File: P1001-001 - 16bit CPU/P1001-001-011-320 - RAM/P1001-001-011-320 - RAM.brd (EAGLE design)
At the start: 200 x 100 mm, 46 parts, among them IC1 74ALS21D, IC10 74ALS08D, IC2 74283D, IC27 MEGA8535-A, IC3 74ALS04D, IC4 74ALS02D, IC5 74LS32D, IC6 74283D, IC7 74283D, IC8 74283D, IC9 74LS32D

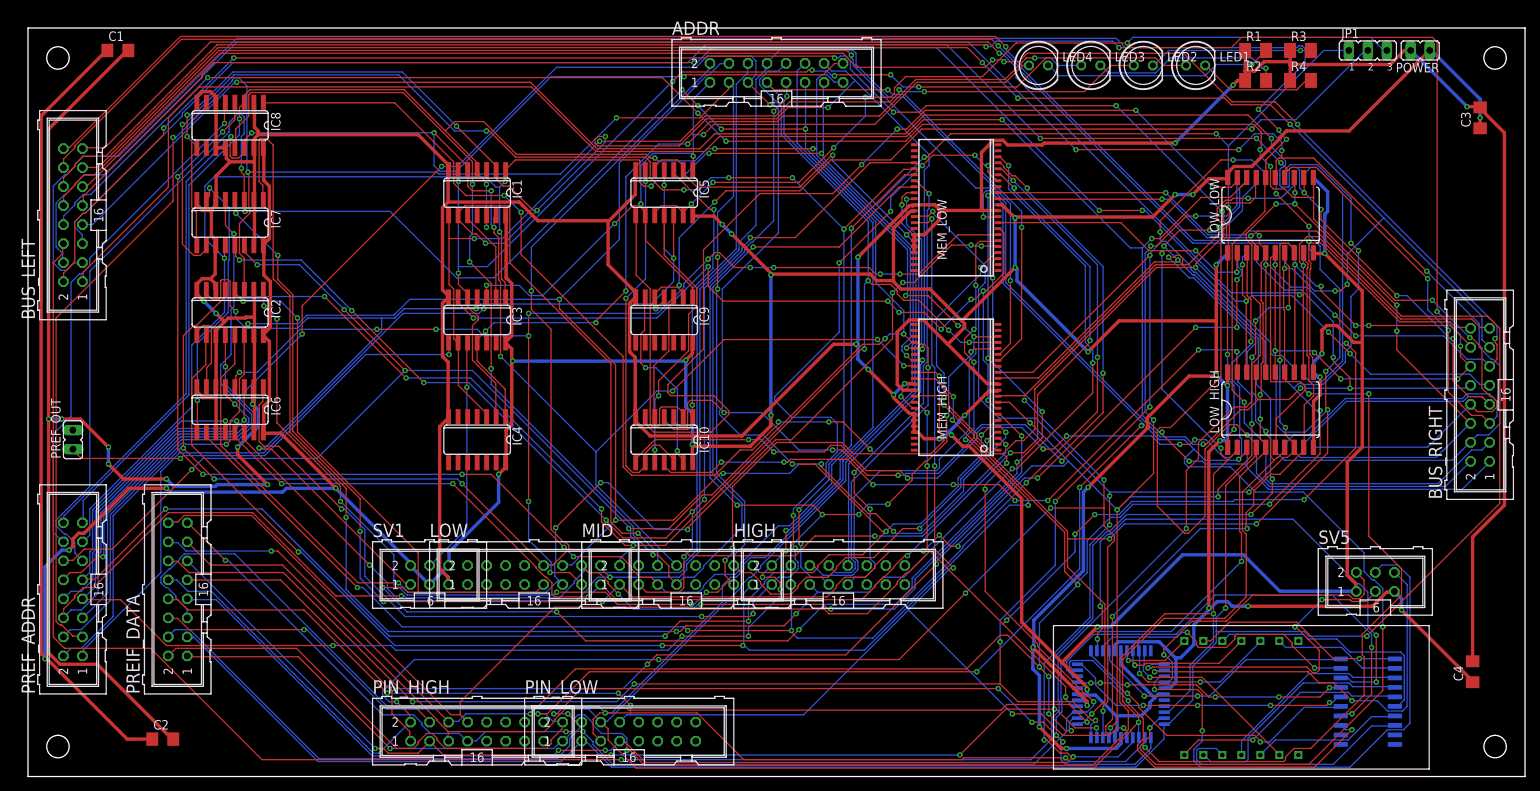
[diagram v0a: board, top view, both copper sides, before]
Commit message: Add the prototype stuff
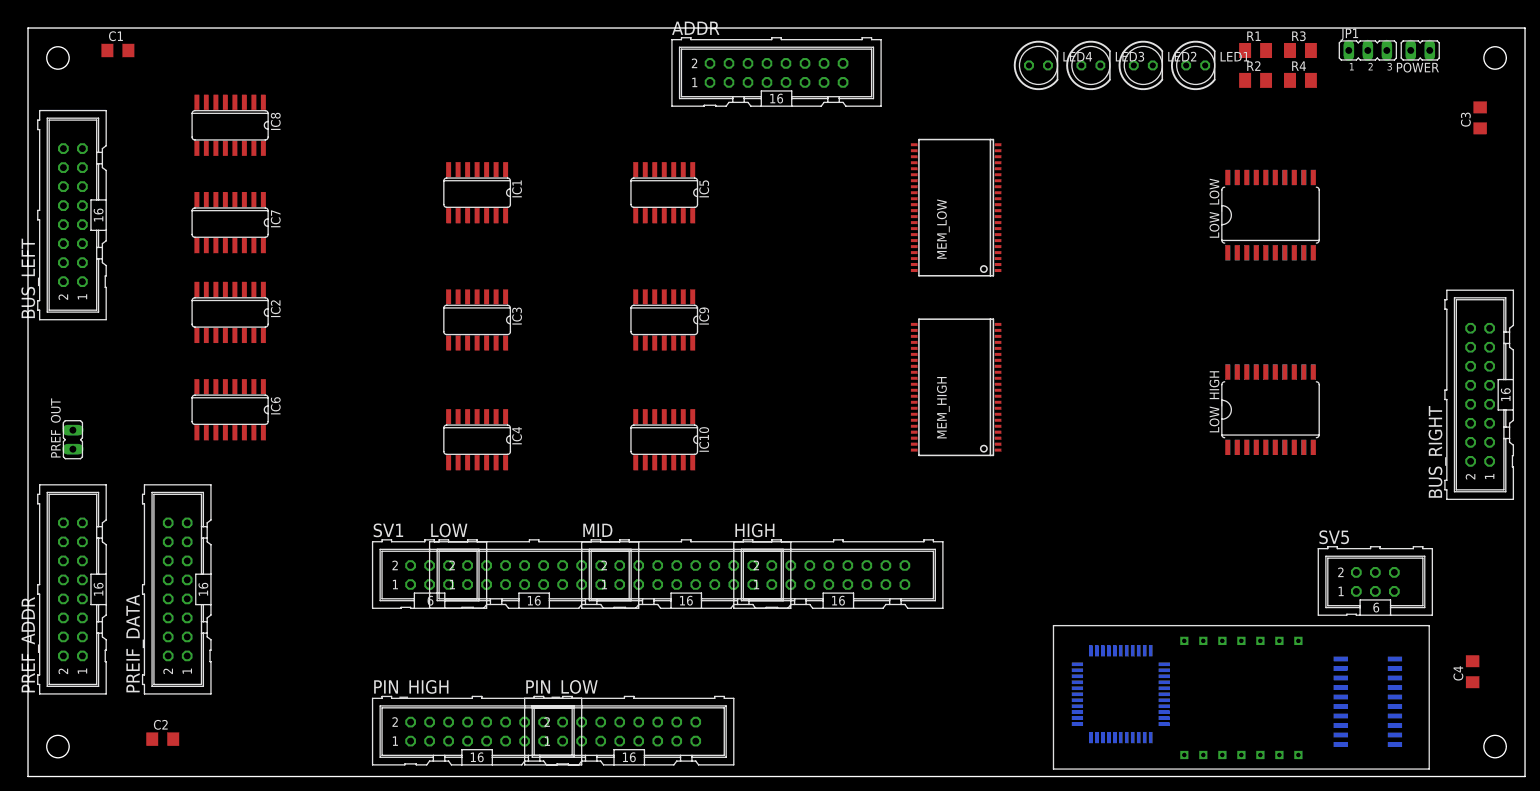
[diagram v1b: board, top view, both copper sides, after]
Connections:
- removed net LOWADDR1: IC2.4, LOW.9, MEM_LOW.3
- removed net LOWADDR10: HIGH.5, IC7.1, MEM_LOW.20
- removed net LOWADDR11: IC7.13, MEM_LOW.26, MID.3
- removed net LOWADDR12: HIGH.7, IC7.10, MEM_LOW.27
- removed net LOWADDR13: IC8.4, MEM_LOW.28, MID.5
- removed net LOWADDR14: HIGH.9, IC8.1, MEM_LOW.29
- removed net LOWADDR15: IC8.13, MEM_LOW.30, MID.7
- removed net LOWADDR2: IC2.1, MEM_LOW.4, MID.13
- removed net LOWADDR3: IC2.13, LOW.11, MEM_LOW.5
- removed net LOWADDR4: IC2.10, MEM_LOW.6, MID.15
- removed net LOWADDR5: IC6.4, LOW.13, MEM_LOW.7
- removed net LOWADDR6: HIGH.1, IC6.1, MEM_LOW.16
- removed net LOWADDR7: IC6.13, LOW.15, MEM_LOW.17
- removed net LOWADDR8: HIGH.3, IC6.10, MEM_LOW.18
- removed net LOWADDR9: IC7.4, MEM_LOW.19, MID.1
- new net HIGHADDR1: IC2.4, LOW.9, MEM_HIGH.3
- new net HIGHADDR10: HIGH.5, IC7.1, MEM_HIGH.20
- new net HIGHADDR11: IC7.13, MEM_HIGH.26, MID.3
- new net HIGHADDR12: HIGH.7, IC7.10, MEM_HIGH.27
- new net HIGHADDR13: IC8.4, MEM_HIGH.28, MID.5
- new net HIGHADDR14: HIGH.9, IC8.1, MEM_HIGH.29
- new net HIGHADDR15: IC8.13, MEM_HIGH.30, MID.7
- new net HIGHADDR2: IC2.1, MEM_HIGH.4, MID.13
- new net HIGHADDR3: IC2.13, LOW.11, MEM_HIGH.5
- new net HIGHADDR4: IC2.10, MEM_HIGH.6, MID.15
- new net HIGHADDR5: IC6.4, LOW.13, MEM_HIGH.7
- new net HIGHADDR6: HIGH.1, IC6.1, MEM_HIGH.16
- new net HIGHADDR7: IC6.13, LOW.15, MEM_HIGH.17
- new net HIGHADDR8: HIGH.3, IC6.10, MEM_HIGH.18
- new net HIGHADDR9: IC7.4, MEM_HIGH.19, MID.1
- net ADDR1: now also MEM_LOW.3; no longer MEM_HIGH.3
- net ADDR10: now also MEM_LOW.20; no longer MEM_HIGH.20
- net ADDR11: now also MEM_LOW.26; no longer MEM_HIGH.26
- net ADDR12: now also MEM_LOW.27; no longer MEM_HIGH.27
- net ADDR13: now also MEM_LOW.28; no longer MEM_HIGH.28
- net ADDR14: now also MEM_LOW.29; no longer MEM_HIGH.29
- net ADDR15: now also MEM_LOW.30; no longer MEM_HIGH.30
- net ADDR2: now also MEM_LOW.4; no longer MEM_HIGH.4
- net ADDR3: now also MEM_LOW.5; no longer MEM_HIGH.5
- net ADDR4: now also MEM_LOW.6; no longer MEM_HIGH.6
- net ADDR5: now also MEM_LOW.7; no longer MEM_HIGH.7
- net ADDR6: now also MEM_LOW.16; no longer MEM_HIGH.16
- net ADDR7: now also MEM_LOW.17; no longer MEM_HIGH.17
- net ADDR8: now also MEM_LOW.18; no longer MEM_HIGH.18
- net ADDR9: now also MEM_LOW.19; no longer MEM_HIGH.19
- net ODD_ADDR: now also IC27.44
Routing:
- net GND: track 893.0 -> 0.00 mm, vias 26 -> 0
- net VCC: track 780.6 -> 0.00 mm, vias 30 -> 0
- net DATA_BUS4: track 369.4 -> 0.00 mm, vias 6 -> 0
- net DATA_BUS1: track 356.2 -> 0.00 mm, vias 9 -> 0
- net EXTERN_BUS5: track 352.5 -> 0.00 mm, vias 7 -> 0
- net DATA_BUS2: track 332.4 -> 0.00 mm, vias 4 -> 0
- net DATA_BUS5: track 318.3 -> 0.00 mm, vias 7 -> 0
- net ADDR13: track 312.3 -> 0.00 mm, vias 10 -> 0
- net ADDR2: track 303.1 -> 0.00 mm, vias 7 -> 0
- net DATA_BUS13: track 296.7 -> 0.00 mm, vias 13 -> 0
- net EXTERN_BUS1: track 296.1 -> 0.00 mm, vias 7 -> 0
- net ADDR5: track 295.3 -> 0.00 mm, vias 6 -> 0
- net DATA_BUS12: track 292.8 -> 0.00 mm, vias 10 -> 0
- net DATA_BUS6: track 292.0 -> 0.00 mm, vias 10 -> 0
- net DATA_BUS7: track 291.1 -> 0.00 mm, vias 10 -> 0
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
